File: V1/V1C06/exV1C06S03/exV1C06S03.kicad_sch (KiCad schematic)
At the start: 6 parts

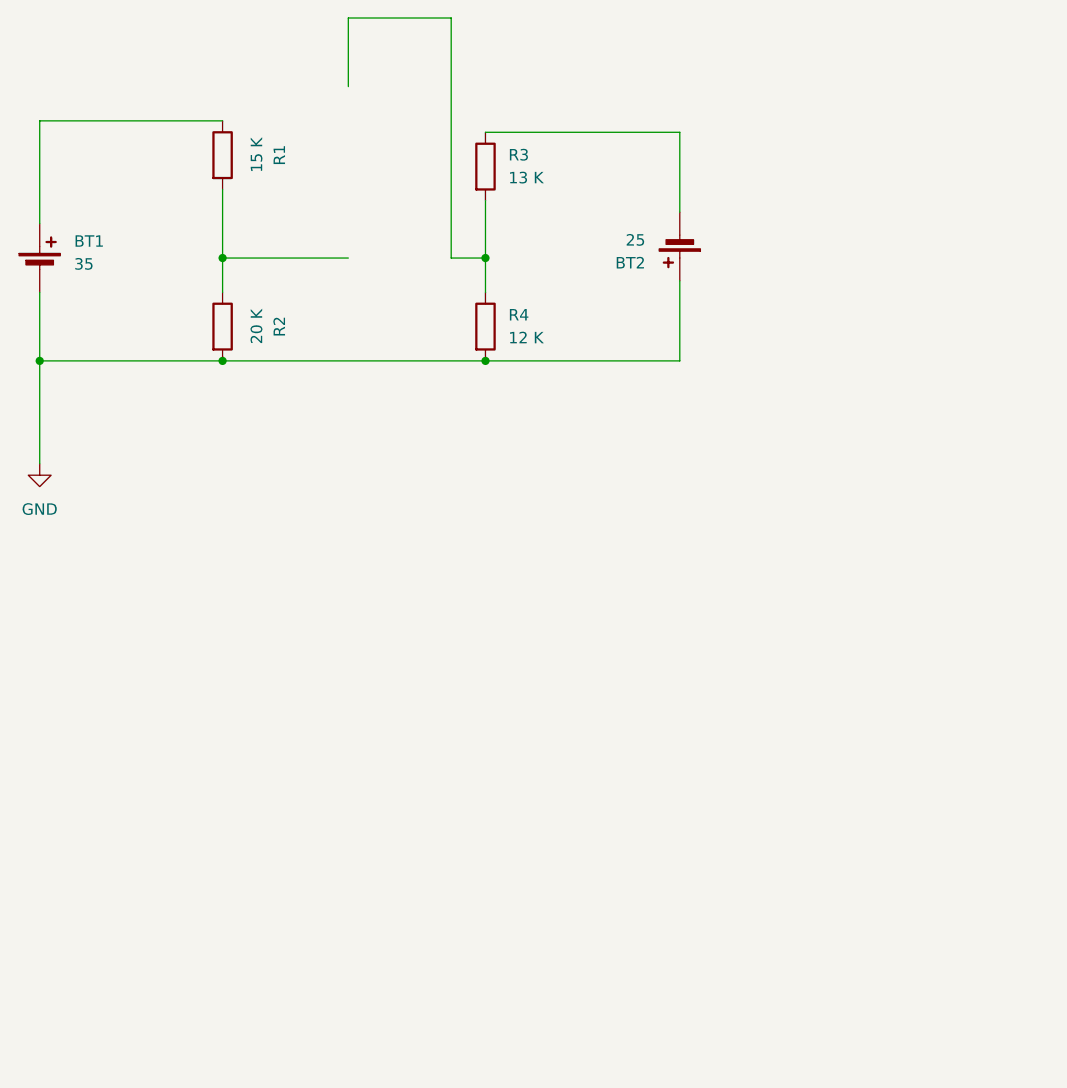
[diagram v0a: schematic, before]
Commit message: upload exV1C06S03
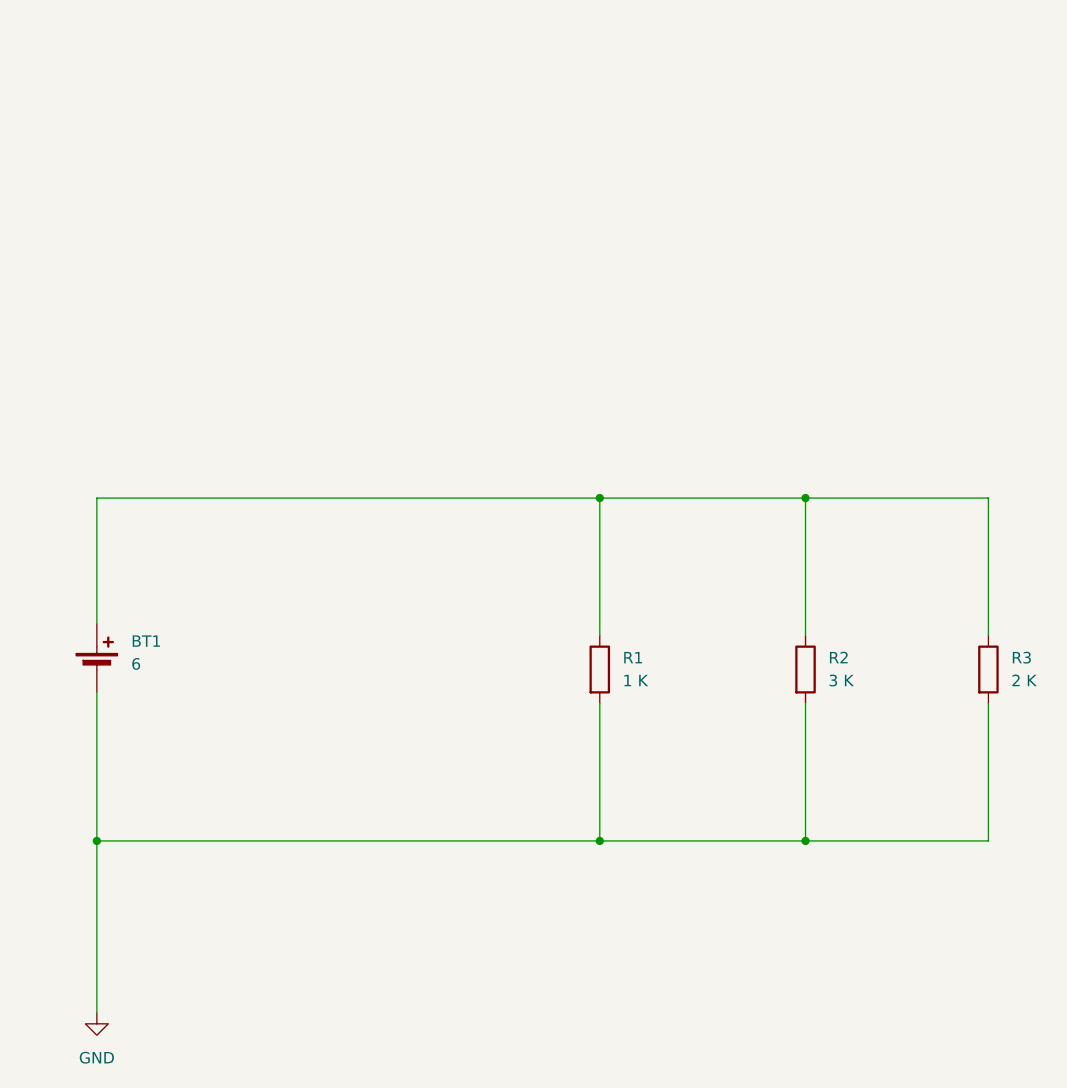
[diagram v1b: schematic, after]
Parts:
- removed BT2: 25, symbol Device:Battery_Cell
- removed R4: 12 K, symbol Device:R
- BT1: value 35 -> 6
- R1: value 15 K -> 1 K
- R2: value 20 K -> 3 K
- R3: value 13 K -> 2 K
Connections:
- net GND: now also R1.2, R3.2
- net at R3.1: now also BT1.1 (+), R1.1, R2.1
